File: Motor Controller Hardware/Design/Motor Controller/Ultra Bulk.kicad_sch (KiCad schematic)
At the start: 35 parts

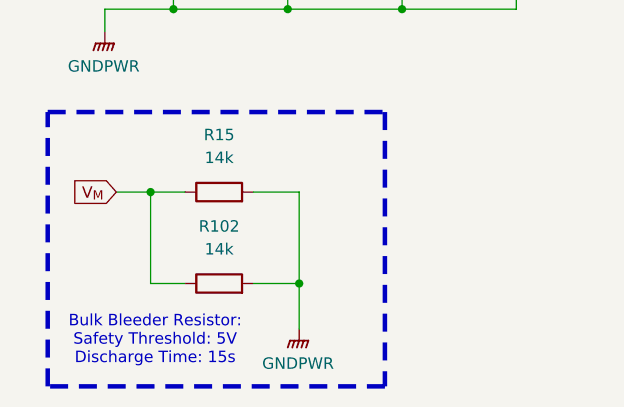
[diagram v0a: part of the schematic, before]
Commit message: A
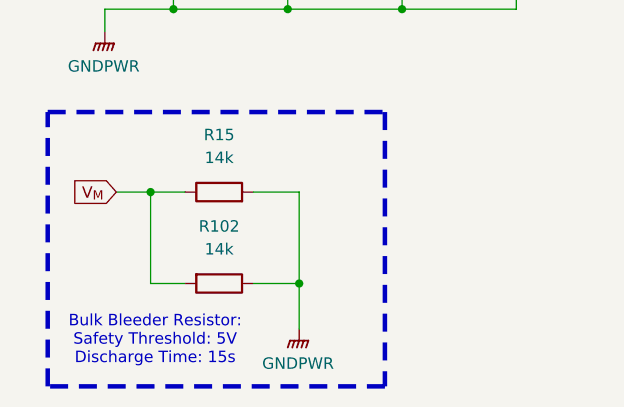
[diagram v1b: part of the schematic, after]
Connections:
- net GNDPWR: now also R102.1; no longer R102.2
- net V_{M}: now also R102.2; no longer R102.1
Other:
- moved on the sheet: R102
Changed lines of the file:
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@@
 	(symbol
 		(lib_id "Device:R")
-		(at 63.5 149.86 90)
+		(at 63.5 149.86 270)
 		(unit 1)
 		(exclude_from_sim no)
@@
 		)
 		(property "Footprint" "Resistor_THT:R_Axial_DIN0617_L17.0mm_D6.0mm_P7.62mm_Vertical"
-			(at 63.5 151.638 90)
+			(at 63.5 148.082 90)
 			(effects
 				(font

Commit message: A
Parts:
- C149, C169, C172, C173, C174, C175, C176, C177, C178, C179, C180, C181, C182, C183, C184, C185, C186, C187, C188, C189, C190, C191, C192, C193, C194, C195, C196, C197, C198: LCSC# (none) -> C5156756
